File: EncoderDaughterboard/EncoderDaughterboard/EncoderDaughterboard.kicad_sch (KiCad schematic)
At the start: 33 parts, among them J1 JST-SH-4, J2 USB_BOOT, J3 RST, Q1 PMOS, U1 RP2040, U2 NCP1117-3.3_SOT223, U3 W25Q128JVS, U4 TMC6300, Y1 Crystal_Small

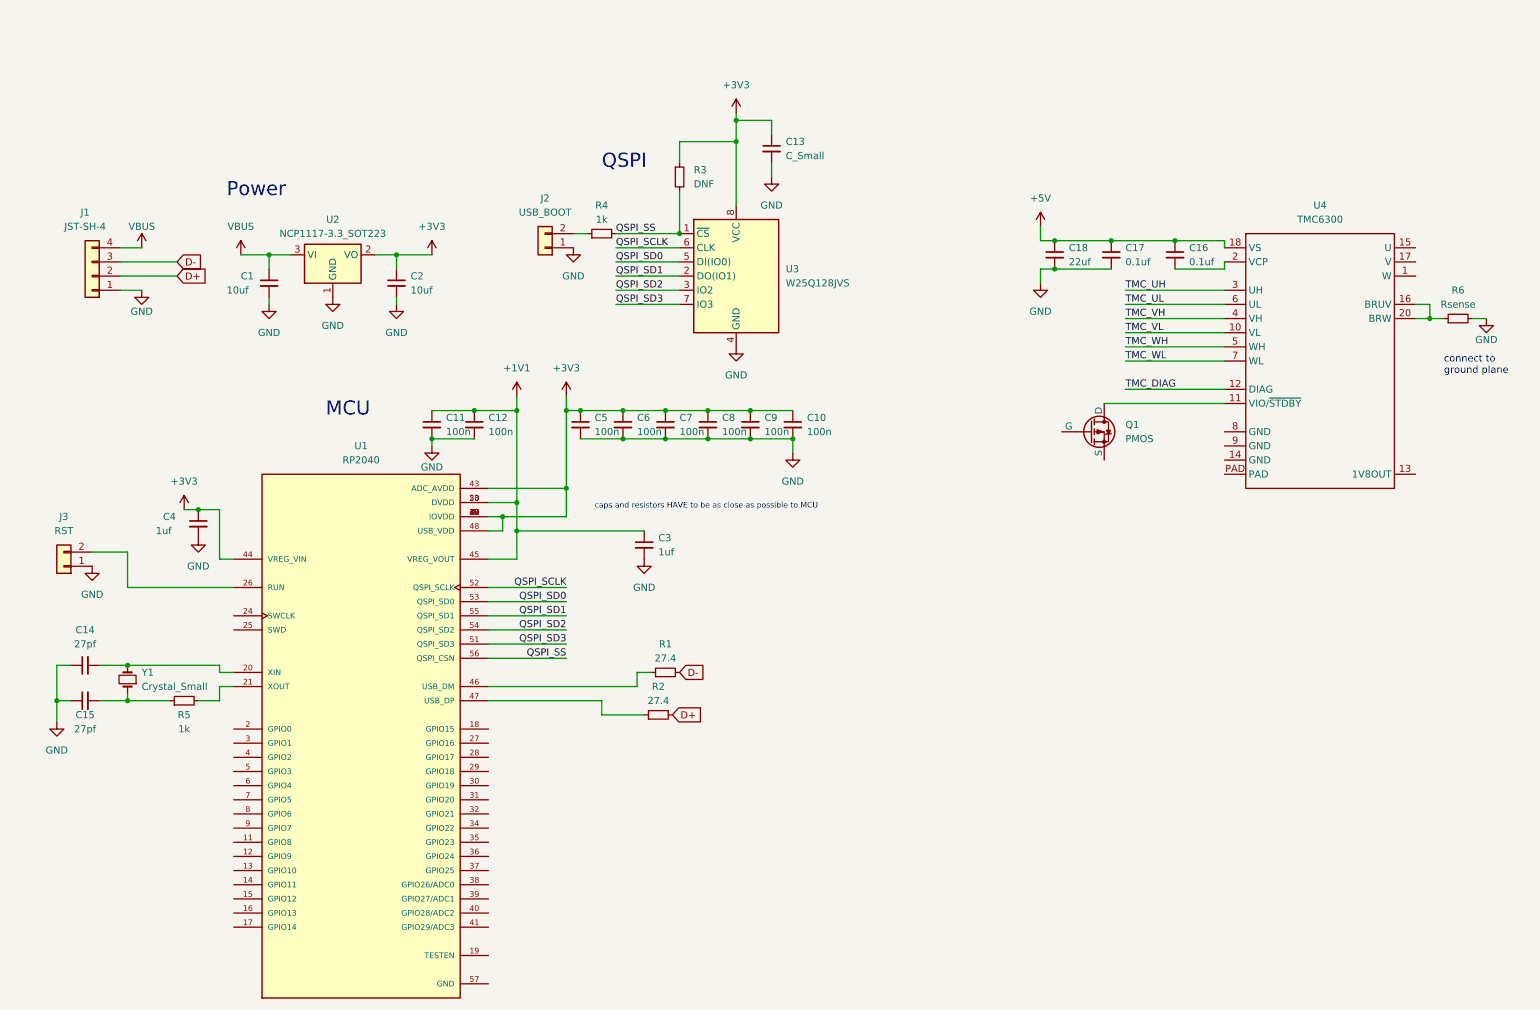
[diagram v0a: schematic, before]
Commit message: encoder daughterboard
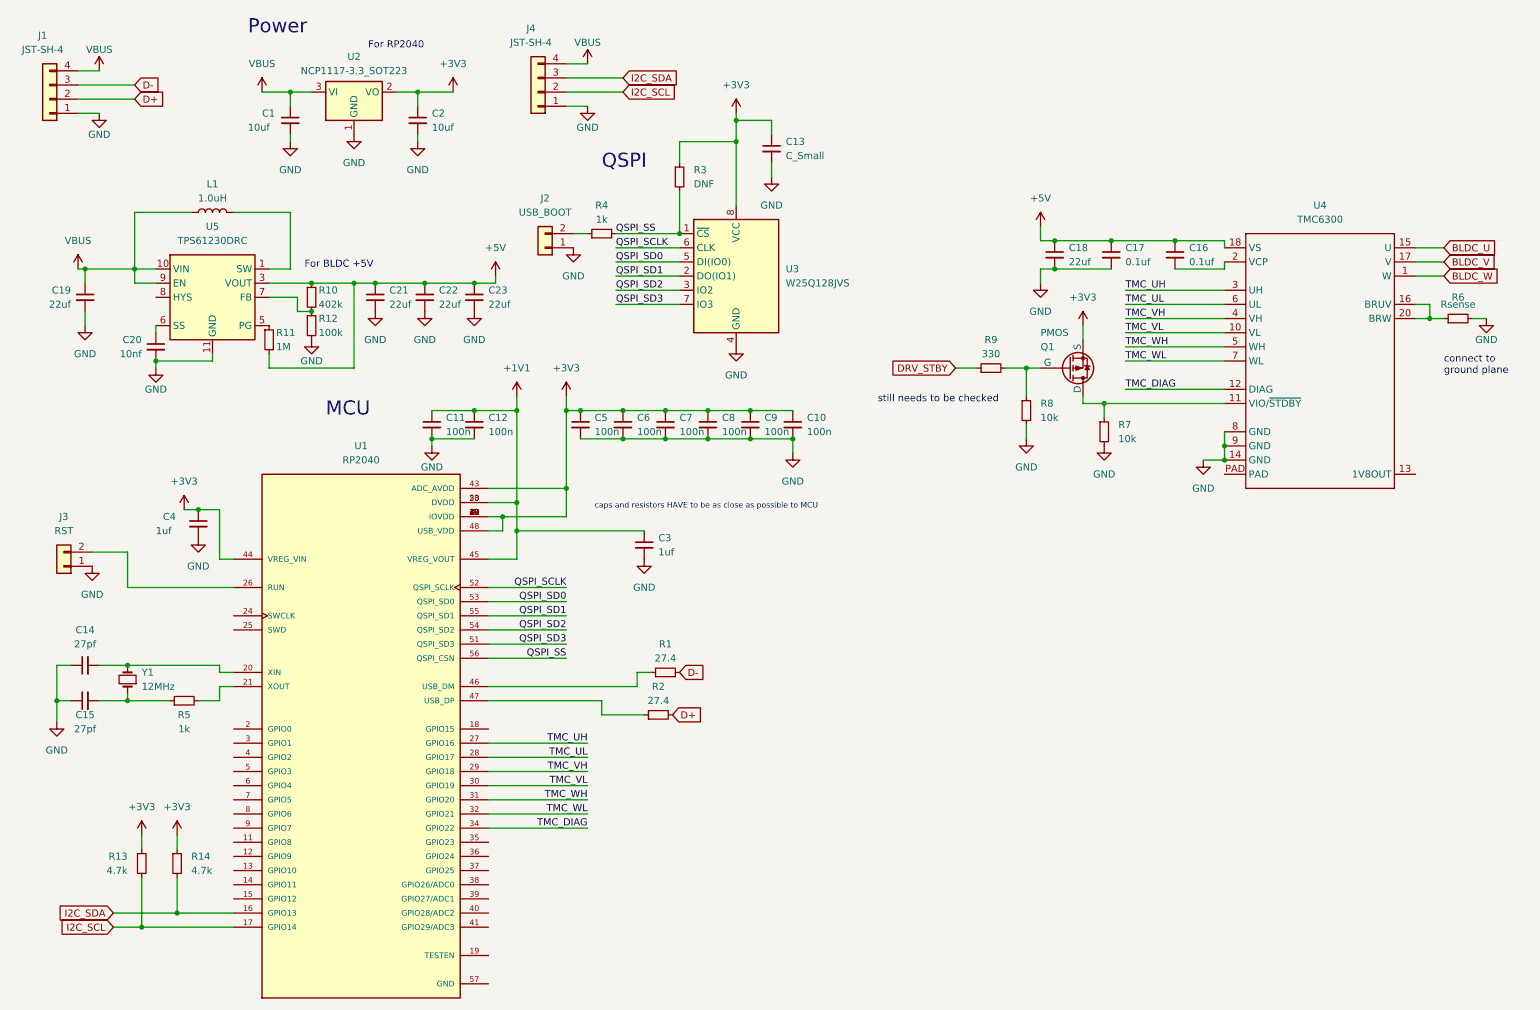
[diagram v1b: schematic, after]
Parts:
- added C19, C21, C22, C23: 22uf, symbol Device:C_Small
- added C20: 10nf, symbol Device:C_Small
- added J4: JST-SH-4, symbol Connector_Generic:Conn_01x04
- added L1: 1.0uH, symbol Device:L
- added R10: 402k, symbol Device:R_Small
- added R11: 1M, symbol Device:R_Small
- added R12: 100k, symbol Device:R_Small
- added R13, R14: 4.7k, symbol Device:R_Small
- added R7, R8: 10k, symbol Device:R_Small
- added R9: 330, symbol Device:R_Small
- added U5: TPS61230DRC, Package_SON:Texas_S-PVSON-N10_ThermalVias, symbol Regulator_Switching:TPS61230DRC
- Y1: value Crystal_Small -> 12MHz
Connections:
- net +3V3: now also Q1.3 (S), R13.1, R14.1
- net +5V: now also C21.1, C22.1, C23.1, R10.1, R11.2, U5.3 (VOUT), U5.4 (VOUT)
- net GND: now also U4.14 (GND), U4.8 (GND), U4.9 (GND), C19.2, C20.2, C21.2, C22.2, C23.2, J4.1 (Pin_1), R12.2, R7.2, R8.2, U5.11 (GND)
- net TMC_DIAG: now also U1.34 (GPIO22)
- net TMC_UH: now also U1.27 (GPIO16)
- net TMC_UL: now also U1.28 (GPIO17)
- net TMC_VH: now also U1.29 (GPIO18)
- net TMC_VL: now also U1.30 (GPIO19)
- net TMC_WH: now also U1.31 (GPIO20)
- net TMC_WL: now also U1.32 (GPIO21)
- net VBUS: now also C19.1, J4.4 (Pin_4), L1.1, U5.10 (VIN), U5.9 (EN)
- net at Q1.1 (D), U4.11 (VIO/~{STDBY}): now also R7.1
- net at Q1.2 (G): now also R8.1, R9.2
- net BLDC_W: now reaches U4.1 (W)
- net BLDC_U: now reaches U4.15 (U)
- net BLDC_V: now reaches U4.17 (V)
- net I2C_SDA: now reaches U1.16 (GPIO13)
- net I2C_SDA: now also J4.3 (Pin_3), R14.2
- net I2C_SCL: now reaches U1.17 (GPIO14)
- net I2C_SCL: now also J4.2 (Pin_2), R13.2
- new net: R10.2, R12.1, U5.7 (FB)
- new net: R11.1, U5.5 (PG)
- new net: C20.1, U5.6 (SS)
- new net: L1.2, U5.1 (SW), U5.2 (SW)
- new net DRV_STBY: R9.1
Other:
- note added: "For BLDC +5V"
- note added: "For RP2040"
- note added: "still needs to be checked"
- moved on the sheet: C1, C2, J1, Q1, U2

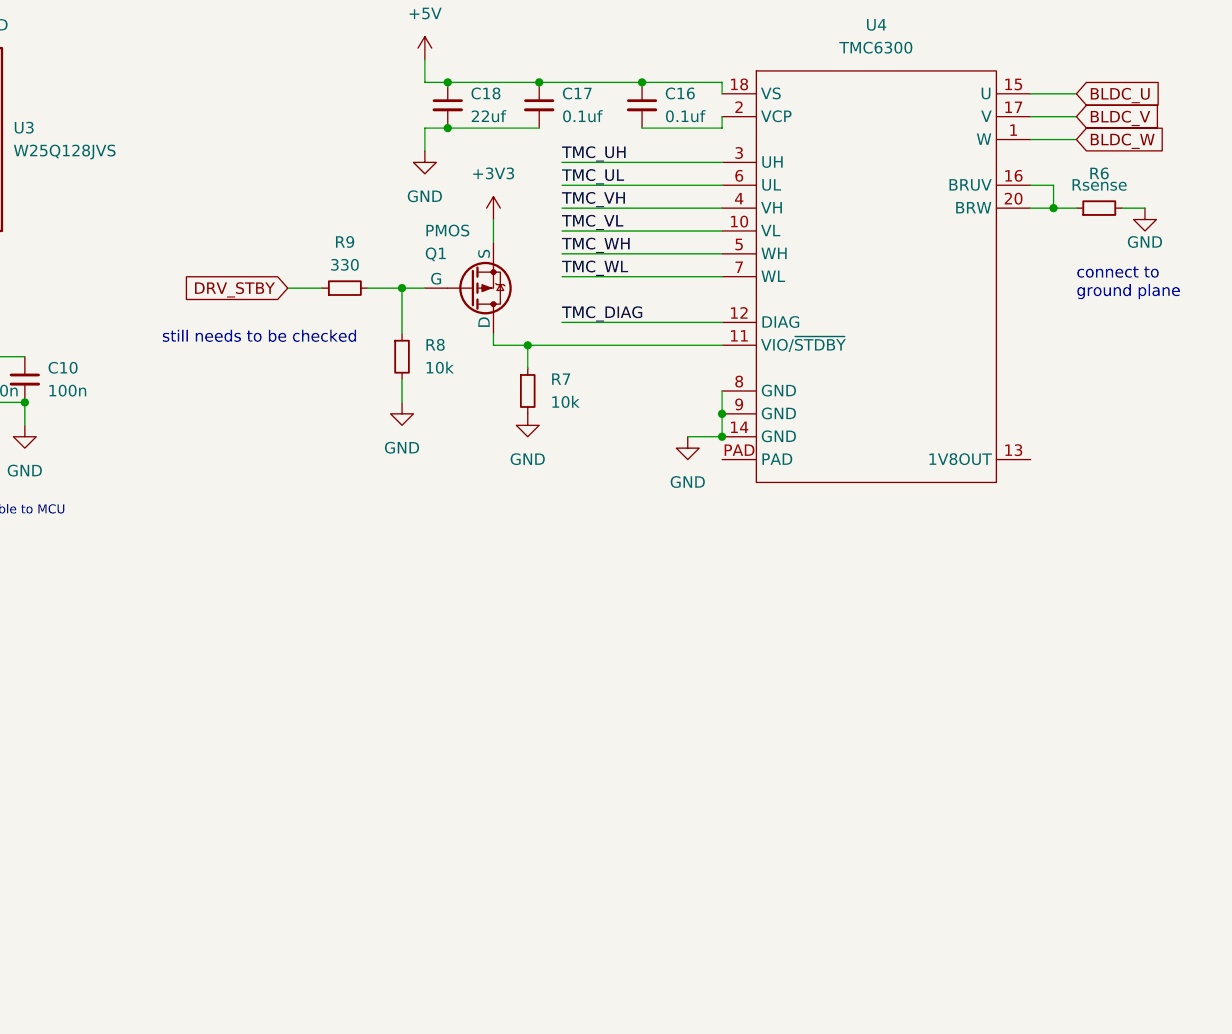
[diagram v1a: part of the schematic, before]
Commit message: Finished Enc. DB Schematic
enter routing hell
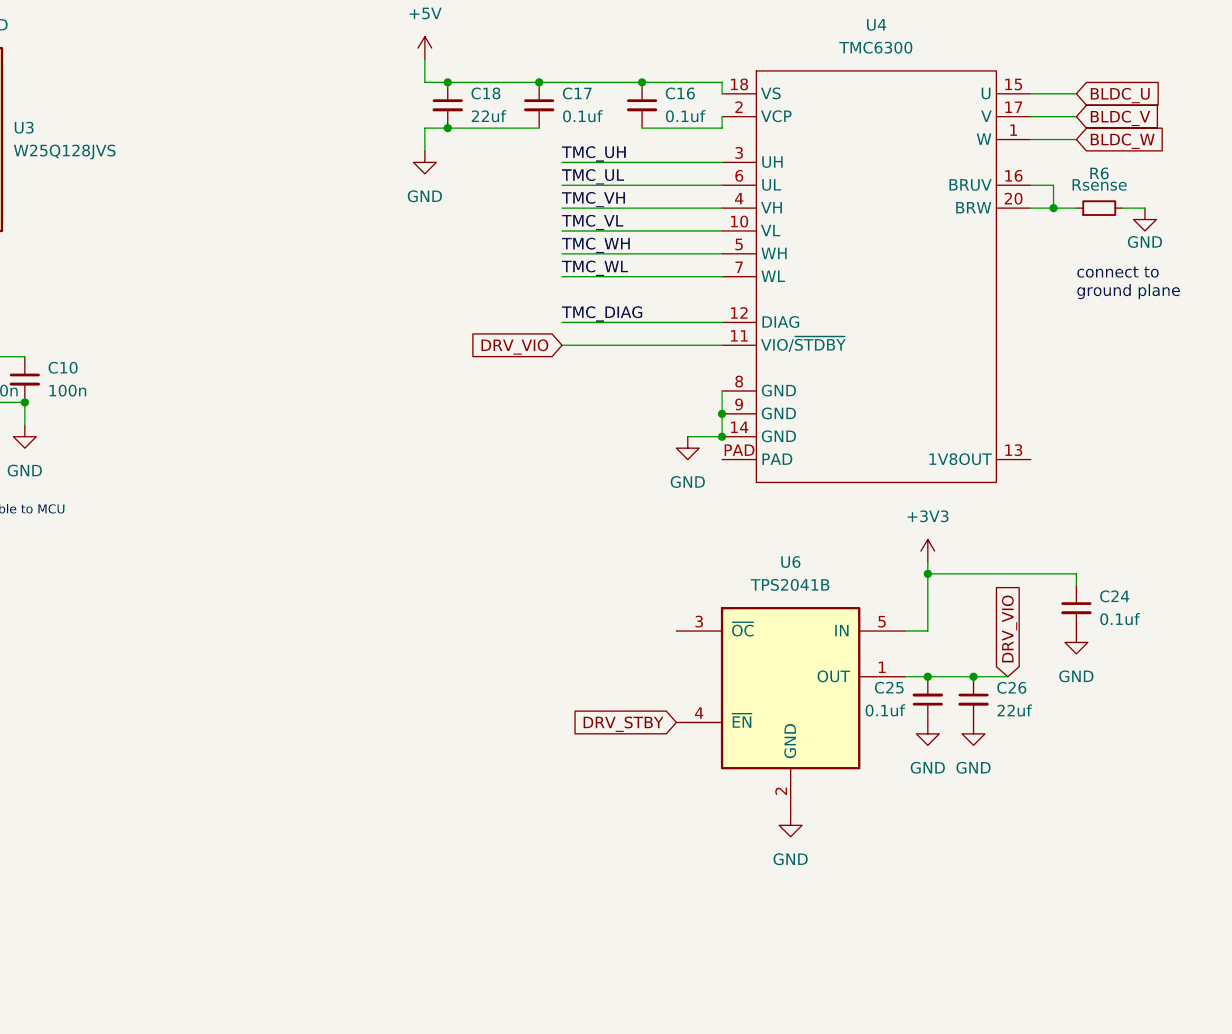
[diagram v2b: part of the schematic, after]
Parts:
- removed Q1: PMOS, symbol Simulation_SPICE:PMOS
- removed R7, R8: 10k, symbol Device:R_Small
- removed R9: 330, symbol Device:R_Small
- added C24, C25: 0.1uf, Capacitor_SMD:C_0402_1005Metric, symbol Device:C_Small
- added C26: 22uf, Capacitor_SMD:C_0402_1005Metric, symbol Device:C_Small
- added U6: TPS2041B, Package_TO_SOT_SMD:SOT-23-5, symbol Power_Management:TPS2041B
- C1, C10, C11, C12, C13, C14, C15, C16, C17, C18, C19, C2, C20, C21, C22, C23, C3, C4, C5, C6, C7, C8, C9: footprint (none) -> Capacitor_SMD:C_0402_1005Metric
- J1, J4: footprint (none) -> Connector_JST:JST_SH_BM04B-SRSS-TB_1x04-1MP_P1.00mm_Vertical
- L1: footprint (none) -> Inductor_SMD:L_0805_2012Metric
- R1, R10, R11, R12, R13, R14, R2, R3, R4, R5, R6: footprint (none) -> Resistor_SMD:R_0402_1005Metric
- U4: footprint (none) -> TMC6300:QFN20_3x3_TRI
- Y1: footprint (none) -> Crystal:Crystal_SMD_0603-2Pin_6.0x3.5mm
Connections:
- net +3V3: now also C24.1, U6.5 (IN)
- net DRV_STBY: now also U6.4 (~{EN})
- net GND: now also C24.2, C25.1, C26.2, U6.2 (GND)
- net DRV_VIO: now reaches U4.11 (VIO/~{STDBY})
- net DRV_VIO: now also C25.2, C26.1, U6.1 (OUT)
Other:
- note removed: "still needs to be checked"

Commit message: footprint
footprint
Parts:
- J2, J3: footprint (none) -> Connector_PinHeader_1.00mm:PinHeader_1x02_P1.00mm_Horizontal
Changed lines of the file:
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@@
       (effects (font (size 1.27 1.27)))
     )
-    (property "Footprint" "" (at 110.49 55.88 0)
+    (property "Footprint" "Connector_PinHeader_1.00mm:PinHeader_1x02_P1.00mm_Horizontal" (at 110.49 55.88 0)
       (effects (font (size 1.27 1.27)) hide)
     )
@@
       (effects (font (size 1.27 1.27)))
     )
-    (property "Footprint" "" (at 24.13 113.03 0)
-      (effects (font (size 1.27 1.27)) hide)
-    )
+    (property "Footprint" "Connector_PinHeader_1.00mm:PinHeader_1x02_P1.00mm_Horizontal" (at 24.13 113.03 0)
+      (effects (font (size 1.27 1.27)) hide)
+    )

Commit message: Val pls dxf
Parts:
- U1: footprint RP2040:QFN40P700X700X90-57N -> RP2040D:QFN40P700X700X90-57N
- U4: footprint TMC6300:QFN20_3x3_TRI -> footprints:QFN20_3x3_TRI
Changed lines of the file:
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@@
       (effects (font (size 1.27 1.27)))
     )
-    (property "Footprint" "TMC6300:QFN20_3x3_TRI" (at 236.22 53.34 0)
+    (property "Footprint" "footprints:QFN20_3x3_TRI" (at 236.22 53.34 0)
       (effects (font (size 1.27 1.27)) hide)
     )
@@
       (effects (font (size 1.27 1.27)))
     )
-    (property "Footprint" "RP2040:QFN40P700X700X90-57N" (at 77.47 144.78 0)
+    (property "Footprint" "RP2040D:QFN40P700X700X90-57N" (at 77.47 144.78 0)
       (effects (font (size 1.27 1.27)) (justify bottom) hide)
     )

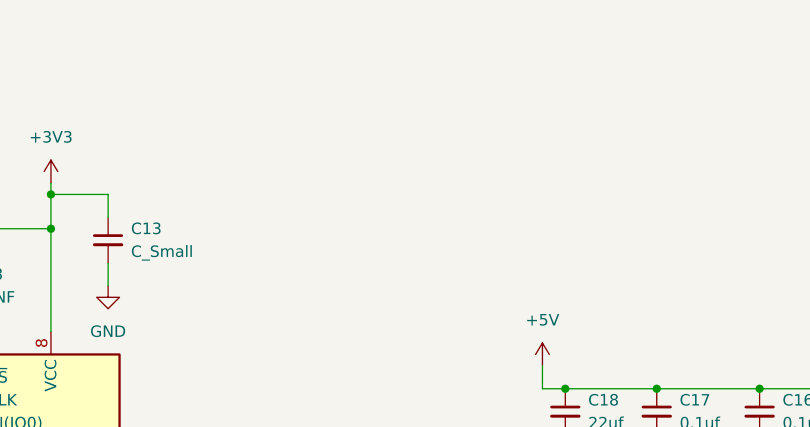
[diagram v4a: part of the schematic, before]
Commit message: over 100 DRC errors but hey weve got a render!
:sleepdepriveddylan:
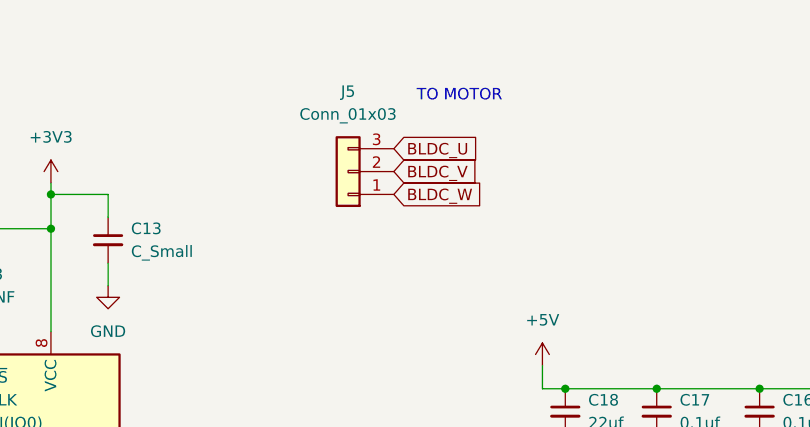
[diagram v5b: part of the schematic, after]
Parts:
- added J5: Conn_01x03, Connector_PinHeader_1.27mm:PinHeader_1x03_P1.27mm_Vertical, symbol Connector_Generic:Conn_01x03
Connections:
- net BLDC_U: now also J5.3 (Pin_3)
- net BLDC_V: now also J5.2 (Pin_2)
- net BLDC_W: now also J5.1 (Pin_1)
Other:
- note added: "TO MOTOR"
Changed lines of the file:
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@@
     (effects (font (size 2.54 2.54)) (justify left bottom))
+  )
+  (text "TO MOTOR\n" (at 185.42 22.86 0)
+    (effects (font (size 1.27 1.27)) (justify left bottom))
   )
   (text "For RP2040" (at 78.74 20.32 0)
@@
     )
   )
+  (global_label "BLDC_U" (shape input) (at 182.88 27.94 0) (fields_autoplaced)
+    (effects (font (size 1.27 1.27)) (justify left))
+    (property "Intersheetrefs" "${INTERSHEET_REFS}" (at 193.0014 27.94 0)
+      (effects (font (size 1.27 1.27)) (justify left) hide)
+    )
+  )
   (global_label "BLDC_W" (shape input) (at 271.78 60.96 0) (fields_autoplaced)
     (effects (font (size 1.27 1.27)) (justify left))
@@
     )
   )
+  (global_label "BLDC_W" (shape input) (at 182.88 33.02 0) (fields_autoplaced)
+    (effects (font (size 1.27 1.27)) (justify left))
+    (property "Intersheetrefs" "${INTERSHEET_REFS}" (at 193.1223 33.02 0)
+      (effects (font (size 1.27 1.27)) (justify left) hide)
+    )
+  )
   (global_label "BLDC_U" (shape input) (at 271.78 55.88 0) (fields_autoplaced)
     (effects (font (size 1.27 1.27)) (justify left))
@@
     (effects (font (size 1.27 1.27)) (justify left))
     (property "Intersheetrefs" "${INTERSHEET_REFS}" (at 135.0652 25.4 0)
+      (effects (font (size 1.27 1.27)) (justify left) hide)
+    )
+  )
+  (global_label "BLDC_V" (shape input) (at 182.88 30.48 0) (fields_autoplaced)
+    (effects (font (size 1.27 1.27)) (justify left))
+    (property "Intersheetrefs" "${INTERSHEET_REFS}" (at 192.7595 30.48 0)
       (effects (font (size 1.27 1.27)) (justify left) hide)
     )
@@
         )
       )
+    )
+  )
+  (symbol (lib_id "Connector_Generic:Conn_01x03") (at 177.8 30.48 180) (unit 1)
+    (in_bom yes) (on_board yes) (dnp no) (fields_autoplaced)
+    (property "Reference" "J5" (at 177.8 21.59 0)
+      (effects (font (size 1.27 1.27)))
+    )
+    (property "Value" "Conn_01x03" (at 177.8 24.13 0)
+      (effects (font (size 1.27 1.27)))
+    )
+    (property "Footprint" "Connector_PinHeader_1.27mm:PinHeader_1x03_P1.27mm_Vertical" (at 177.8 30.48 0)
+      (effects (font (size 1.27 1.27)) hide)
+    )
+    (property "Datasheet" "~" (at 177.8 30.48 0)
+      (effects (font (size 1.27 1.27)) hide)
+    )
+    (pin "1")
+    (pin "2")
+    (pin "3")
+    (instances
+      (project "EncoderDaughterboard"
+        (path "/5265d892-8b8c-462a-bf73-dc9194acd9ae"
+          (reference "J5") (unit 1)
+        )
+      )
